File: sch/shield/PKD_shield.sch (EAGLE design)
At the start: 35 parts, among them IC1 LM393N, IC2 TL084P, IC3 PIC12F683P, IC5 74HCT243N, Q1 BS170

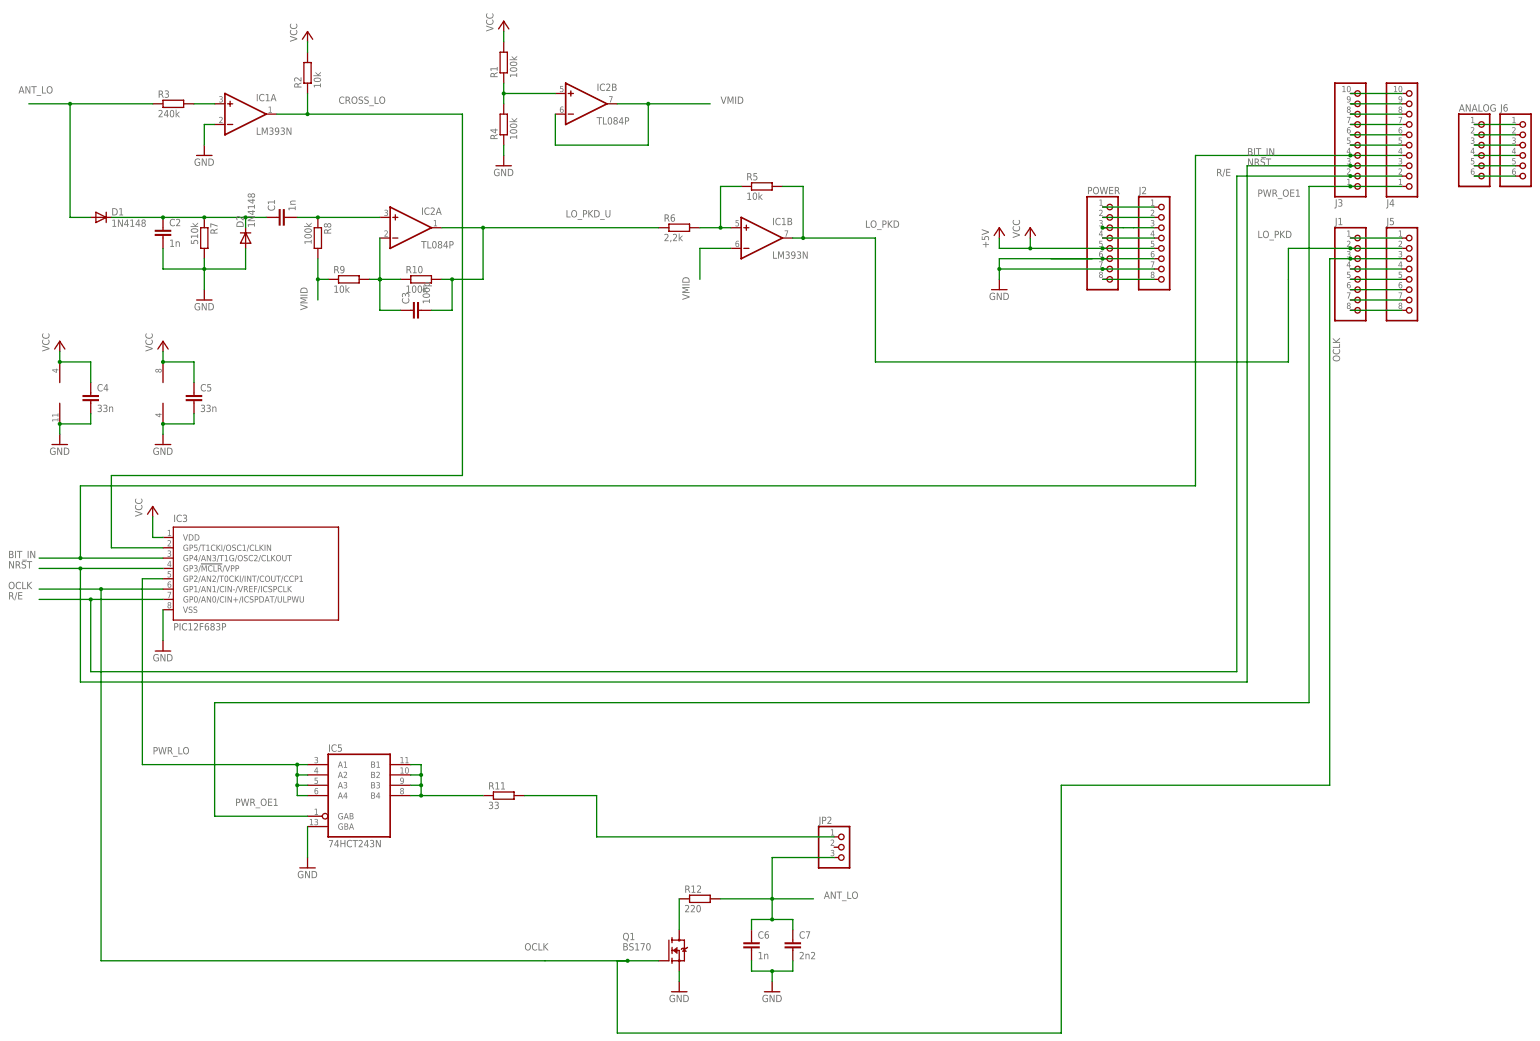
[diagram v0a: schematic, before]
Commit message: Minor update
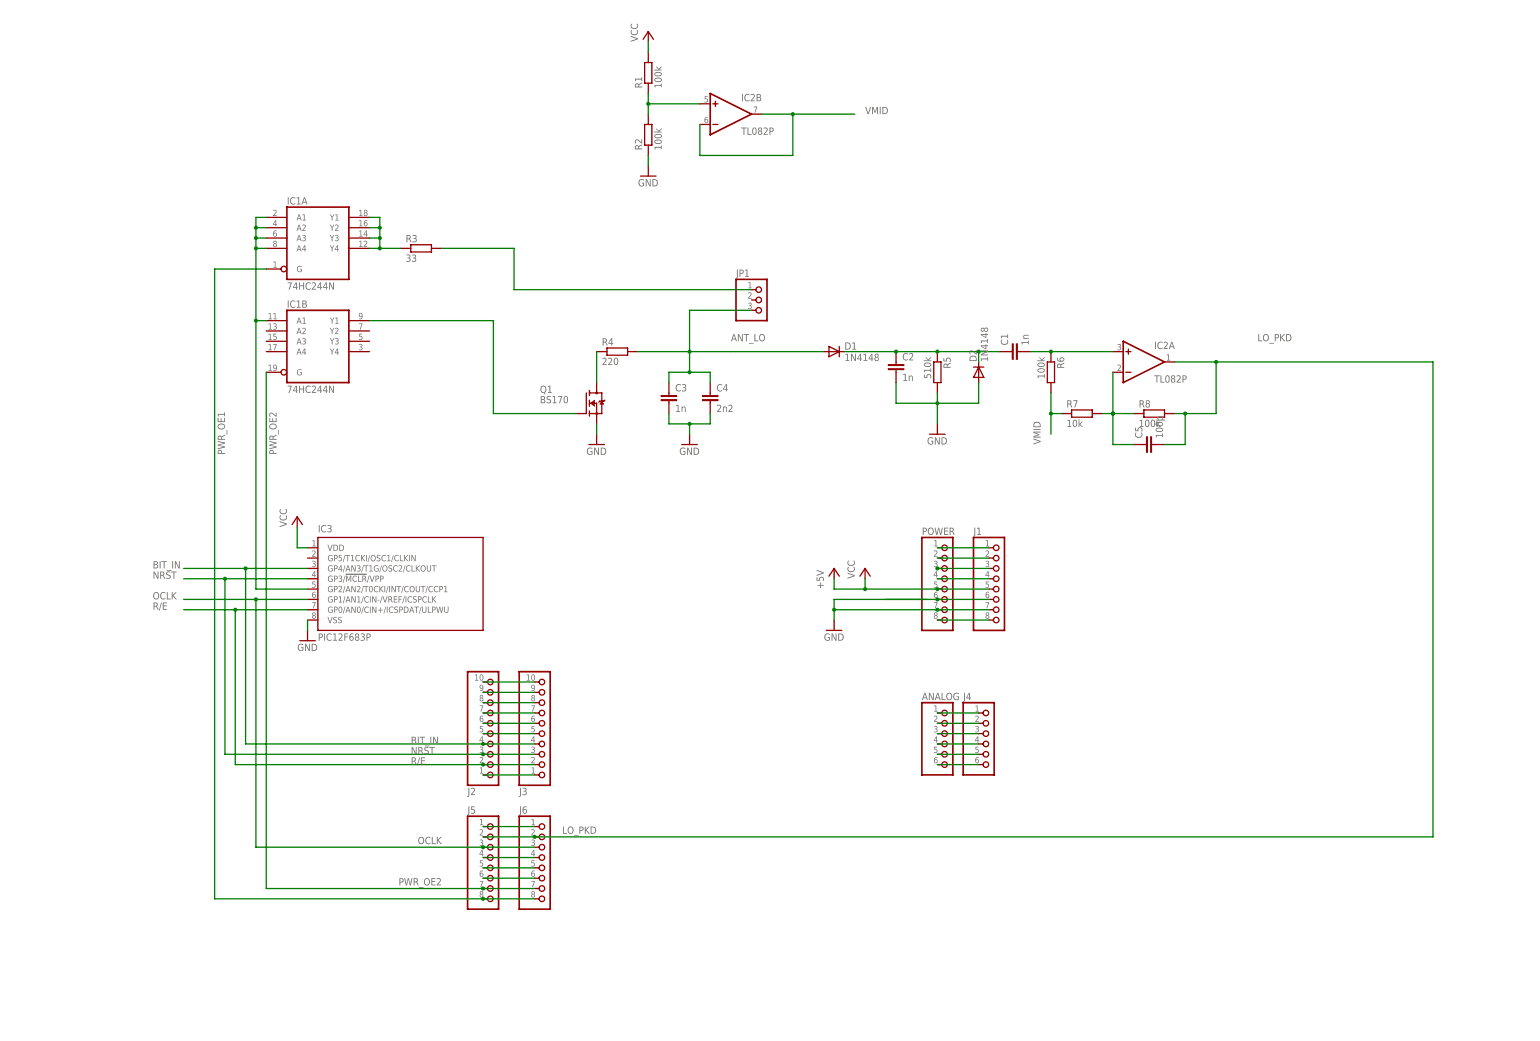
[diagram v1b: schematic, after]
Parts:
- removed C6: 1n, rcl:C-EU025-025X050
- removed C7: 2n2, rcl:C-EU025-025X050
- removed IC5: 74HCT243N, 74xx-eu:74HCT243N
- removed JP2: (no value), pinhead:PINHD-1X3/90
- removed R10: 100k, rcl:R-EU_0207/10
- removed R11: 33, rcl:R-EU_0207/10
- removed R12: 220, rcl:R-EU_0207/10
- removed R9: 10k, rcl:R-EU_0207/10
- added JP1: (no value), pinhead:PINHD-1X3/90
- C2: device rcl:C-EU050-030X075 -> rcl:C-EU025-025X050
- C3: value 100p -> 1n
- C4: value 33n -> 2n2
- C5: value 33n -> 100p
- IC1: value LM393N -> 74HC244N; device linear:LM393N -> 74xx-eu:74HC244N
- IC2: value TL084P -> TL082P; device linear:TL084P -> linear:TL082P
- J2: device SmartPrj:PINHD-1X8TH -> SmartPrj:PINHD-1X10TH
- J4: device SmartPrj:PINHD-1X10TH -> pinhead:PINHD-1X6
- J6: device pinhead:PINHD-1X6 -> SmartPrj:PINHD-1X8TH
- R2: value 10k -> 100k
- R3: value 240k -> 33
- R4: value 100k -> 220
- R5: value 10k -> 510k
- R6: value 2,2k -> 100k
- R7: value 510k -> 10k
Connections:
- removed net CROSS_LO: IC1A.OUT, IC3.GP5/T1CKI/OSC1/CLKIN, R2.1
- removed net LO_PKD_U: C3.2, IC2A.OUT, R10.2, R6.1
- removed net N$14: J1.7, J5.7
- removed net N$15: J1.8, J5.8
- removed net N$28: IC1A.+IN, R3.2
- removed net N$35: IC1B.+IN, R5.1, R6.2
- new net N$2: IC1B.Y1, Q1.G
- new net N$5: J2.1, J3.1
- new net PWR_OE2: IC1B.G, J5.7, J6.7
- net +9V: now also J1.8; no longer J2.8
- net ANT_LO: now also C3.1, C4.1, JP1.3, R4.2; no longer C6.1, C7.1, JP2.3, R12.2, R3.1
- net BIT_IN: now also J2.4; no longer J4.4
- net GND: now also C3.2, J1.7, R2.1, R5.2; no longer C5.2, C6.2, C7.2, IC1A.-IN, IC1P.V-, IC2P.V-, IC5A.GBA, J2.7, R4.1, R7.2
- net LO_PKD: now also C5.2, IC2A.OUT, J6.2, R8.2; no longer IC1B.OUT, J1.2, R5.2
- net N$1: now also J1.3; no longer J2.3
- net N$11: now also J6.4; no longer J1.4
- net N$12: now also J6.5; no longer J1.5
- net N$13: now also J6.6; no longer J1.6
- net N$141: now also J2.9; no longer J4.9
- net N$142: now also J2.10; no longer J4.10
- net N$16: now also R2.2; no longer R4.2
- net N$17: now also R5.1; no longer R7.1
- net N$18: now also J4.1; no longer J6.1
- net N$19: now also J4.2; no longer J6.2
- net N$20: now also J4.3; no longer J6.3
- net N$21: now also J4.4; no longer J6.4
- net N$22: now also J4.5; no longer J6.5
- net N$222: now also J2.8; no longer J4.8
- net N$223: now also J1.4; no longer J2.4
- net N$23: now also J4.6; no longer J6.6
- net N$24: now also J2.7; no longer J4.7
- net N$25: now also J1.6; no longer J2.6
- net N$26: now also R6.1; no longer R8.1
- net N$27: now also C5.1, R7.2, R8.1; no longer C3.1, R10.1, R9.2
- net N$29: now also JP1.1, R3.2; no longer JP2.1, R11.2
- net N$3: now also J2.6; no longer J4.6
- net N$30: now also IC1A.Y1, IC1A.Y2, IC1A.Y3, IC1A.Y4, R3.1; no longer IC5A.B1, IC5A.B2, IC5A.B3, IC5A.B4, R11.1
- net N$31: now also J1.2; no longer J2.2
- net N$32: now also J1.1; no longer J2.1
- net N$34: now also R4.1; no longer R12.1
- net N$4: now also J2.5; no longer J4.5
- net N$8: now also J6.1; no longer J1.1
- net NRST: now also J2.3; no longer J4.3
- net OCLK: now also J6.3; no longer J1.3, Q1.G
- net PWR_LO: now also IC1A.A1, IC1A.A2, IC1A.A3, IC1A.A4, IC1B.A1; no longer IC5A.A1, IC5A.A2, IC5A.A3, IC5A.A4
- net PWR_OE1: now also IC1A.G, J5.8, J6.8; no longer IC5A.GAB, J3.1, J4.1
- net R/E: now also J2.2; no longer J4.2
- net VCC: now also J1.5; no longer C4.1, C5.1, IC1P.V+, IC2P.V+, J2.5, R2.2
- net VMID: now also R6.2, R7.1; no longer IC1B.-IN, R8.2, R9.1
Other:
- moved on the sheet: ANALOG, C1, C2, C3, C4, C5, D1, D2, IC2A, IC2B, IC3, J1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
